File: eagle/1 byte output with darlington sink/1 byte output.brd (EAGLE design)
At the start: 85.1 x 44.1 mm, 26 parts, among them IC1 74LS165N, IC2 74LS165N, X3 MKDSN1,5/8-5,08, X5 MKDSN1,5/8-5,08

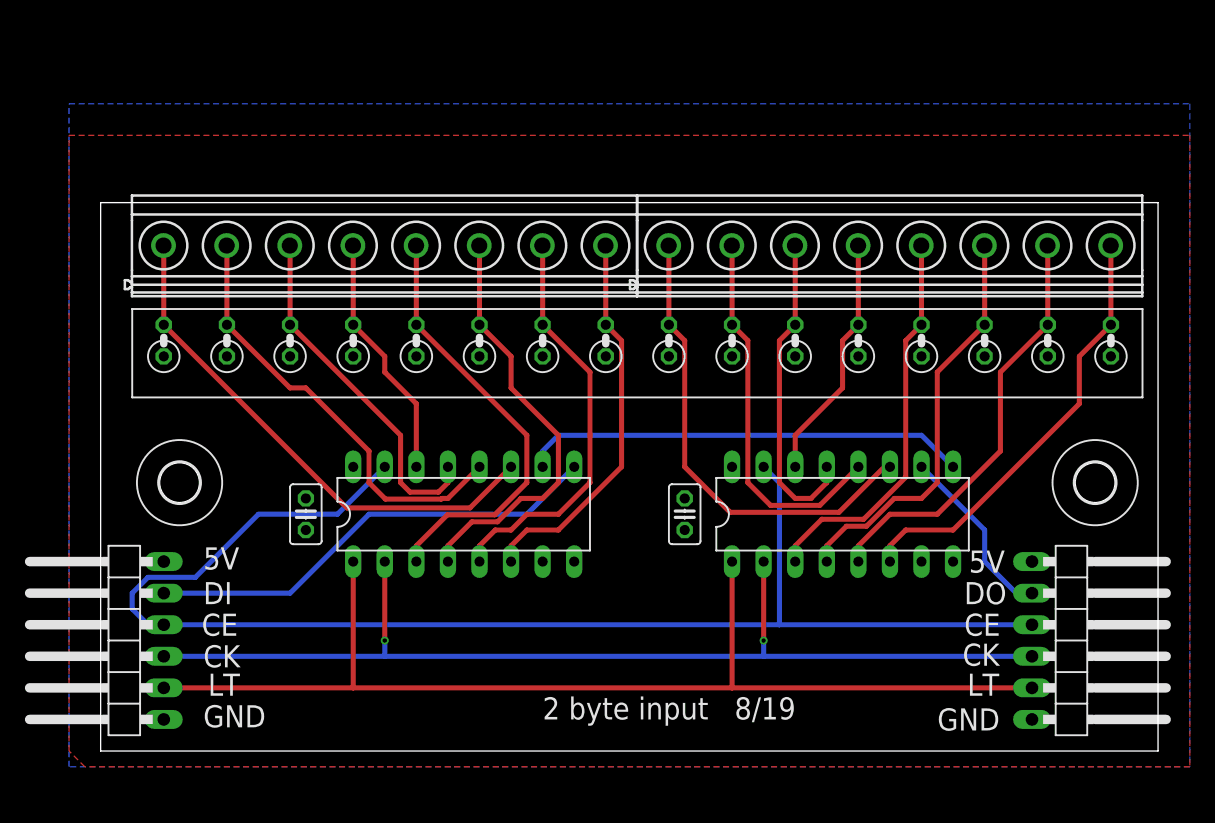
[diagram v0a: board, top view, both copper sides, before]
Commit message: periodic check-in
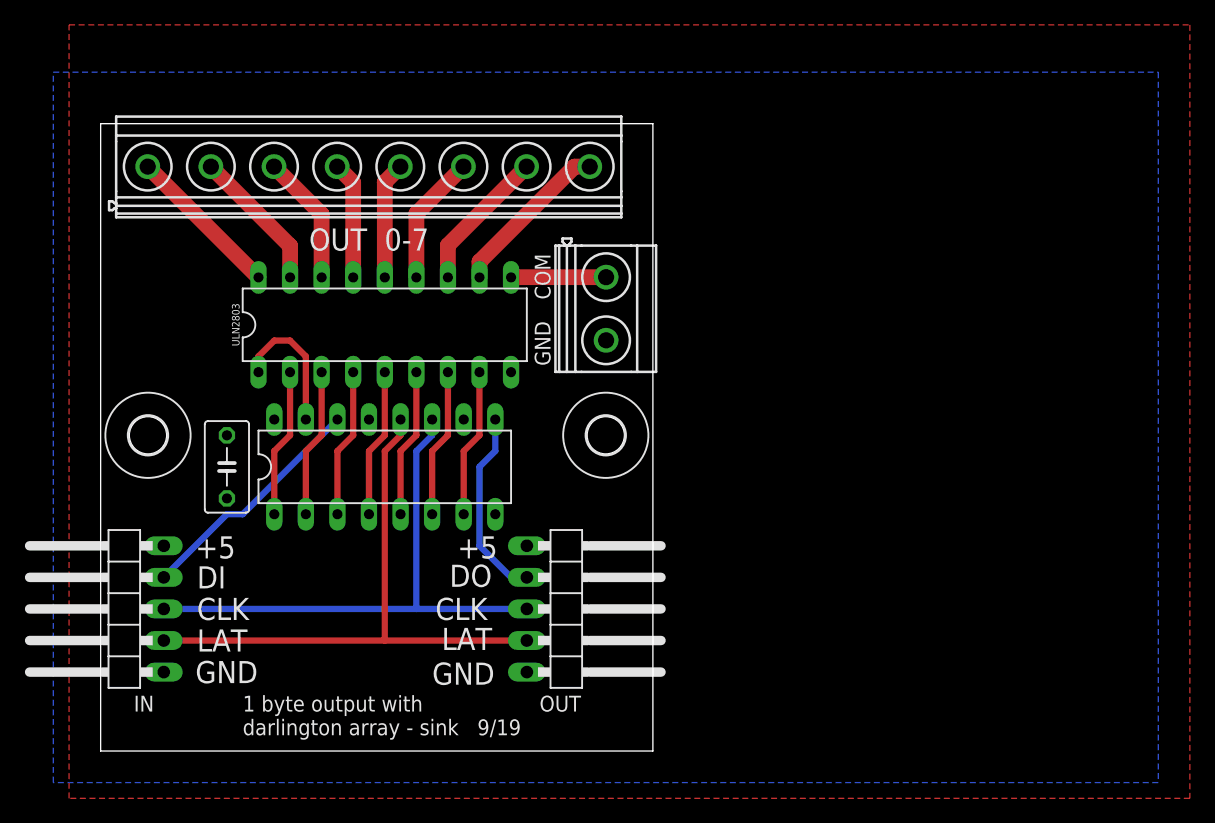
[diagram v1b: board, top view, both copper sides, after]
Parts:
- removed C1: 0.1uf, resistor:C025-025X050
- removed IC2: 74LS165N, 74xx-us:DIL16
- removed R1, R10, R11, R12, R13, R14, R15, R16, R2, R3, R4, R5, R6, R7, R8: (no value), resistor:0207/2V
- removed R9: 4K7, resistor:0207/2V
- removed X3: MKDSN1,5/8-5,08, con-phoenix-508:MKDSN1,5/8-5,08
- added ULN2803: (no value), SparkFun-IC-Special-Function:DIL18
- added X1: MKDSN1,5/8-5,08, con-phoenix-508:MKDSN1,5/8-5,08
- C2: value 0.1uf -> (none); device resistor:C025-025X050 -> resistor:C050-035X075
- H1, H2: value MOUNT-HOLE3.2 -> MOUNT-HOLE3.0; device holes:3,2 -> holes:3,0
- IC1: value 74LS165N -> 74LS595N
- JP1, JP2: device pinhead:1X06/90 -> pinhead:1X05/90
- X5: value MKDSN1,5/8-5,08 -> MKDSN1,5/2-5,08; device con-phoenix-508:MKDSN1,5/8-5,08 -> con-phoenix-508:MKDSN1,5/2-5,08
- moved JP2 77.5 mm to (1.27, 11.4), turned to 90 degrees
- moved H2 39.6 mm to (40.6, 25.4)
- moved C2 37.0 mm to (10.2, 22.9)
- moved JP1 36.9 mm to (38.1, 11.4), turned to 270 degrees
- moved X5 23.4 mm to (40.6, 35.6), turned to 270 degrees
- moved IC1 7.41 mm to (22.9, 22.9)
- moved H1 4.58 mm to (3.81, 25.4)
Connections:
- removed net +5V: C1.1, C2.1, IC1.16, IC2.16, JP1.6, JP2.1, R1.1, R10.1, R11.1, R12.1, R13.1, R14.1, R15.1, R16.1, R2.1, R3.1, R4.1, R5.1, R6.1, R7.1, R8.1, R9.1
- removed net CE: IC1.15, IC2.15, JP1.4, JP2.3
- removed net INA0: IC1.11, R1.2, X3.1
- removed net INA1: IC1.12, R2.2, X3.2
- removed net INA2: IC1.13, R3.2, X3.3
- removed net INA3: IC1.14, R4.2, X3.4
- removed net INA4: IC1.3, R5.2, X3.5
- removed net INA5: IC1.4, R6.2, X3.6
- removed net INA6: IC1.5, R7.2, X3.7
- removed net INA7: IC1.6, R8.2, X3.8
- removed net INB0: IC2.11, R9.2, X5.1
- removed net INB1: IC2.12, R10.2, X5.2
- removed net INB2: IC2.13, R11.2, X5.3
- removed net INB3: IC2.14, R12.2, X5.4
- removed net INB4: IC2.3, R13.2, X5.5
- removed net INB5: IC2.4, R14.2, X5.6
- removed net INB6: IC2.5, R15.2, X5.7
- removed net INB7: IC2.6, R16.2, X5.8
- removed net S0: IC1.9, JP1.5
- removed net S1: IC1.10, IC2.9
- removed net SX: IC2.10, JP2.2
- new net COM: ULN2803.10, X5.1
- new net DI: IC1.14, JP2.4
- new net DO: IC1.9, JP1.2
- new net N$1: ULN2803.18, X1.1
- new net N$2: ULN2803.17, X1.2
- new net N$3: ULN2803.16, X1.3
- new net N$4: ULN2803.15, X1.4
- new net N$5: ULN2803.14, X1.5
- new net N$6: ULN2803.13, X1.6
- new net N$7: ULN2803.12, X1.7
- new net N$8: ULN2803.11, X1.8
- new net OUT0: IC1.15, ULN2803.1
- new net OUT1: IC1.1, ULN2803.2
- new net OUT2: IC1.2, ULN2803.3
- new net OUT3: IC1.3, ULN2803.4
- new net OUT4: IC1.4, ULN2803.5
- new net OUT5: IC1.5, ULN2803.6
- new net OUT6: IC1.6, ULN2803.7
- new net OUT7: IC1.7, ULN2803.8
- new net VCC: C2.1, IC1.10, IC1.16, JP1.1, JP2.5
- net CLK: now also IC1.11, JP2.3; no longer IC1.2, IC2.2, JP2.4
- net GND: now also IC1.13, JP1.5, JP2.1, ULN2803.9, X5.2; no longer C1.2, IC2.8, JP1.1, JP2.6
- net LATCH: now also IC1.12, JP1.4, JP2.2; no longer IC1.1, IC2.1, JP1.2, JP2.5
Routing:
- net CE: track 111.9 -> 0.00 mm
- net LATCH: track 90.2 -> 47.5 mm
- net INA0: track 41.8 -> 0.00 mm
- net CLK: track 85.1 -> 45.0 mm, vias 2 -> 0
- net INB0: track 37.9 -> 0.00 mm
- net S0: track 37.2 -> 0.00 mm
- net S1: track 35.9 -> 0.00 mm
- net INA1: track 35.1 -> 0.00 mm
- net INB7: track 35.0 -> 0.00 mm
- net INA4: track 35.0 -> 0.00 mm
- net INB6: track 34.0 -> 0.00 mm
- net INA5: track 34.0 -> 0.00 mm
- net INB5: track 32.9 -> 0.00 mm
- net INA6: track 32.9 -> 0.00 mm
- net INB4: track 31.6 -> 0.00 mm
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- added copper zone on layer 1, net VCC
- removed copper zone on layer 1, net +5V
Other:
- board size 85.1 x 44.1 mm -> 44.4 x 50.5 mm
- board text added: "+5"
- board text added: "1 byte output with darlington array - sink 9/19"
- board text added: "CLK"
- board text added: "COM"
- board text added: "IN"
- board text added: "LAT"
- board text added: "OUT"
- board text added: "OUT 0-7"
- board text removed: "2 byte input 8/19"
- board text removed: "5V"
- board text removed: "CE"
- board text removed: "CK"
- board text removed: "LT"
